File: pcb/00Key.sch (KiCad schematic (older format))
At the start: 2 parts, among them Q1 IRLZ44N, U1 Teensy4.1

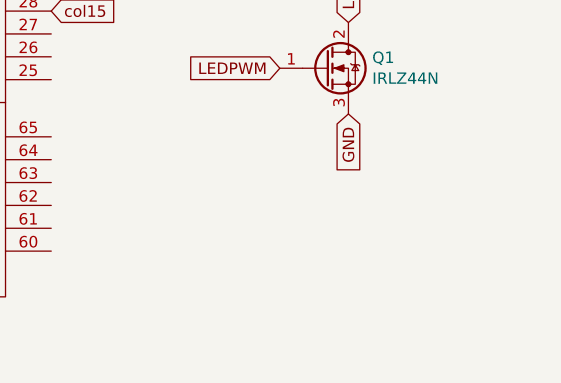
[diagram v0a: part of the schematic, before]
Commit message: oled
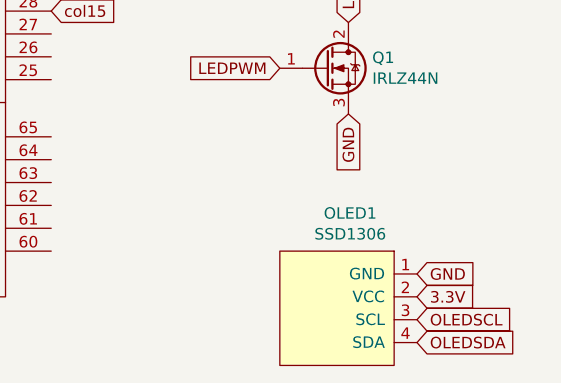
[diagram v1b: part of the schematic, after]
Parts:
- added OLED1: SSD1306, oled:128x64OLED, symbol oled:SSD1306
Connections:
- net 3.3V: now also OLED1.2 (VCC)
- net GND: now also OLED1.1 (GND)
- net OLEDSCL: now also OLED1.3 (SCL)
- net OLEDSDA: now also OLED1.4 (SDA)
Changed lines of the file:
@@
 Text GLabel 5200 2550 2    50   Input ~ 0
 LEDGND
+$Comp
+L oled:SSD1306 OLED1
+U 1 1 5F70EDBF
+P 4750 4550
+F 0 "OLED1" V 4335 4608 50  0000 C CNN
+F 1 "SSD1306" V 4426 4608 50  0000 C CNN
+F 2 "oled:128x64OLED" H 4750 4800 50  0001 C CNN
+F 3 "" H 4750 4800 50  0001 C CNN
+	1    4750 4550
+	0    1    1    0
+$EndComp
+Text GLabel 5100 4400 2    50   Input ~ 0
+GND
+Text GLabel 5100 4500 2    50   Input ~ 0
+3.3V
+Text GLabel 5100 4600 2    50   Input ~ 0
+OLEDSCL
+Text GLabel 5100 4700 2    50   Input ~ 0
+OLEDSDA
 $EndSCHEMATC
